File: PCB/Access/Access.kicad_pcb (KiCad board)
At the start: 2 copper layers, 70 x 70 mm, 85 parts, among them J1 USB-C, J2 RFID, J3 INPUTS, J4 USB-PROG, J5 POWER, J6 DOOR2, J7 DOOR1, J8 Shelly, Q2 PMF250XNEX, SW1 ESE13V01A, U1 MD8942, U10 ESP32-S3-MINI-1, U2 MD8942, U3 G3VM-41GR8, U8 G3VM-41GR8

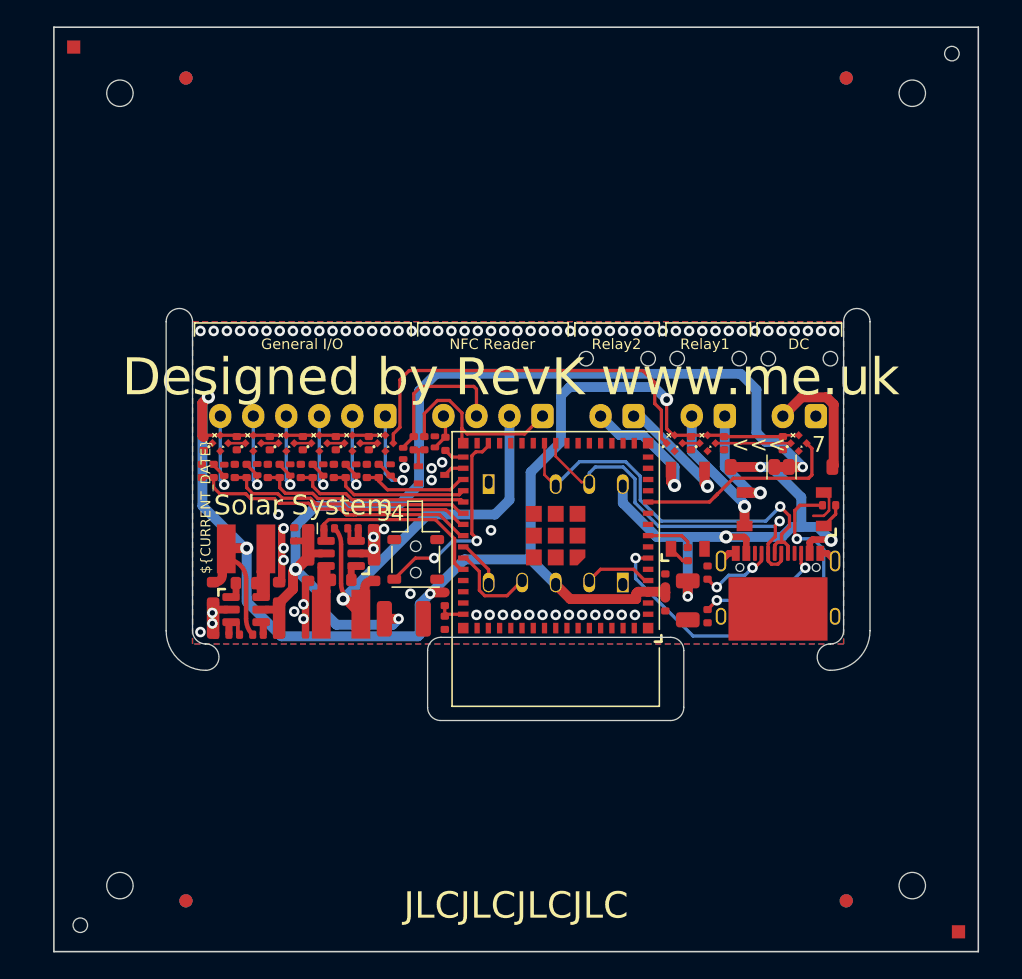
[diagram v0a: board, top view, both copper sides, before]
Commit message: Tidy
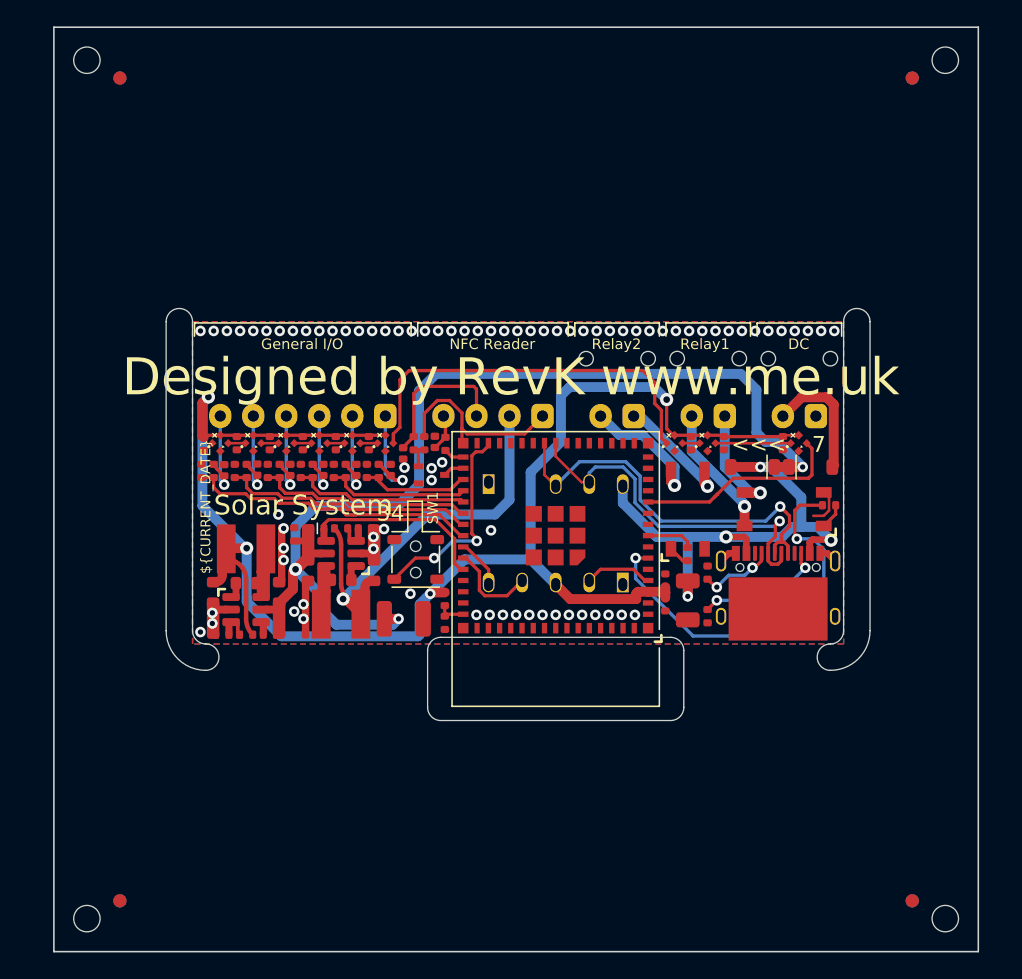
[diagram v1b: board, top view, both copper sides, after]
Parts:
- moved J1 1.39 mm to (119.8, 105.9)
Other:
- copper layers 2 -> 4
- board text removed: "15"
- board text removed: "16"
- board text removed: "17"
- board text removed: "18"
- board text removed: "19"
- board text removed: "21"
- board text removed: "22"
- board text removed: "23"
